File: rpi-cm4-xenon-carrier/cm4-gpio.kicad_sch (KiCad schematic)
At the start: 22 parts

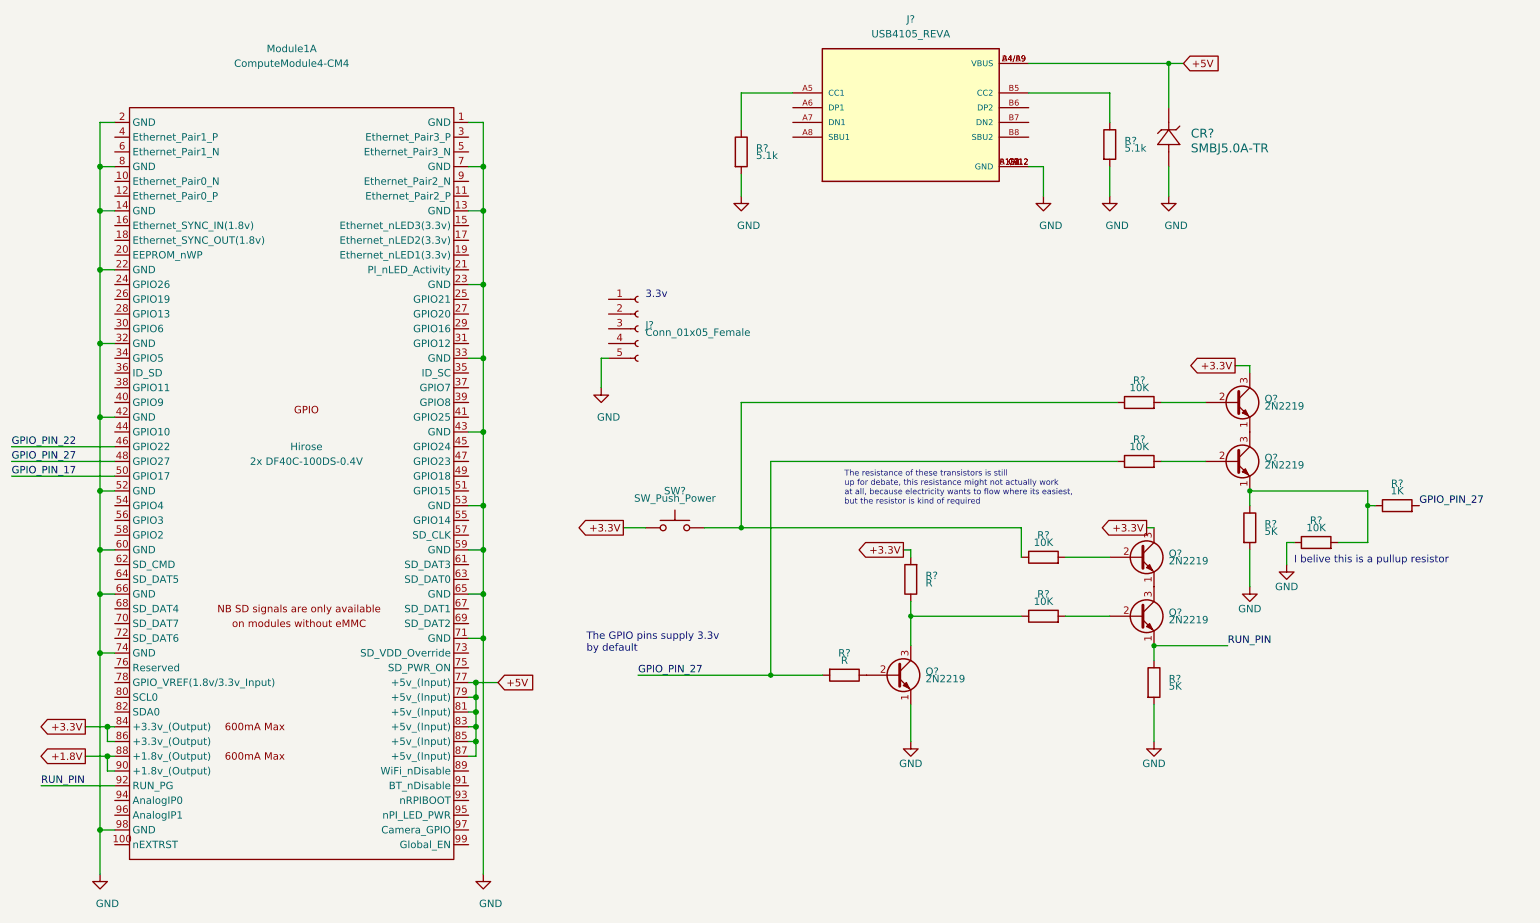
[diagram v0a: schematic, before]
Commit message: RP2040
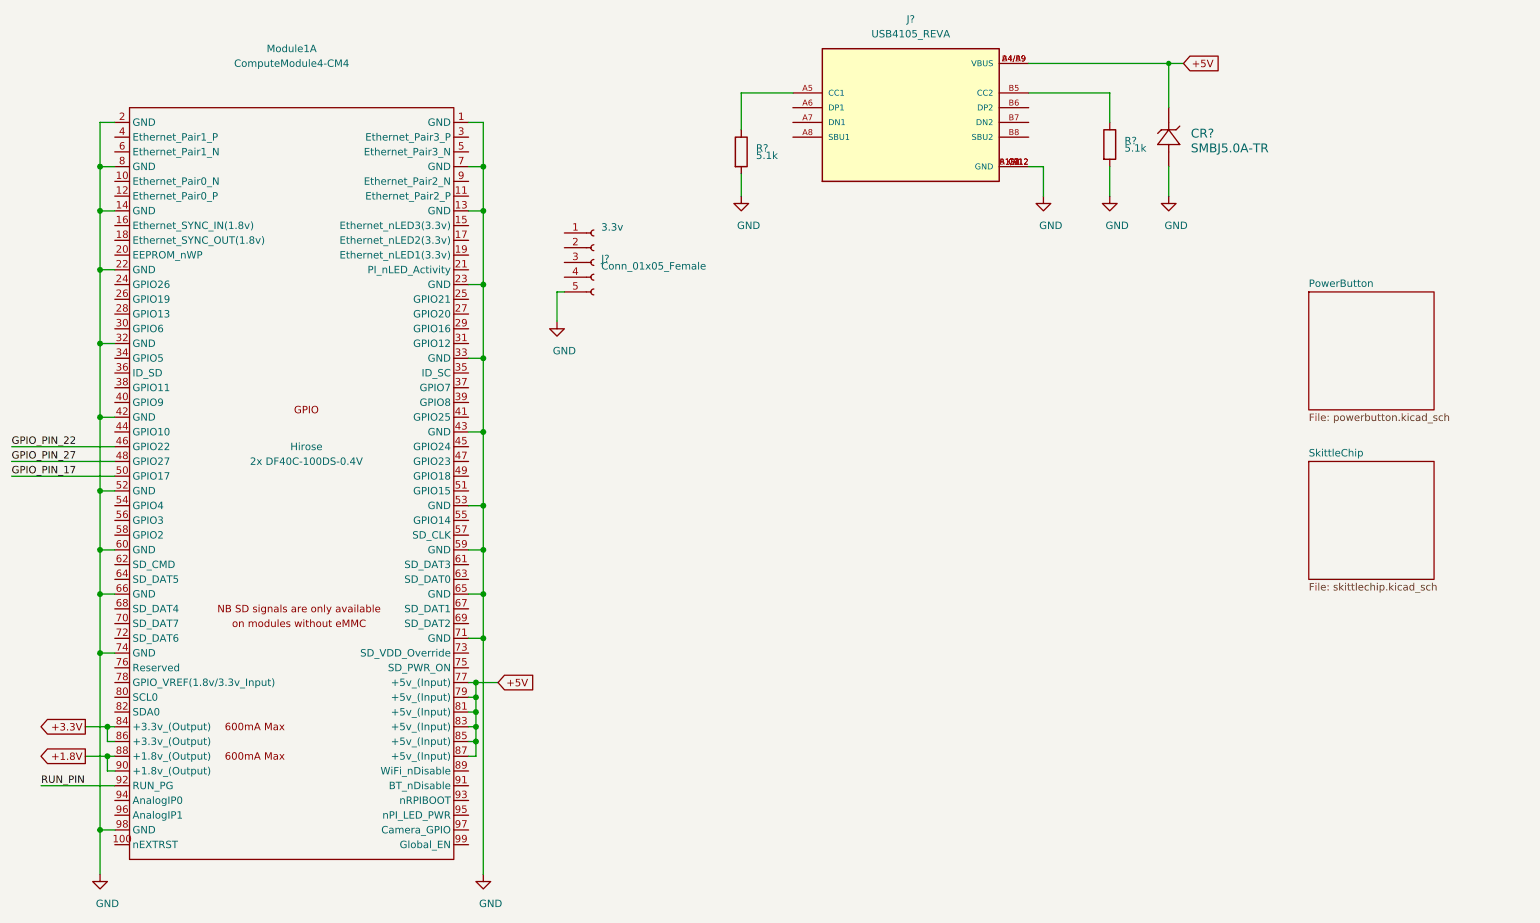
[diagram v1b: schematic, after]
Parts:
- removed Q? (x5): 2N2219, Package_TO_SOT_THT:TO-39-3, symbol Transistor_BJT:2N2219
- removed R? (x5): 10K, symbol Device:R
- removed R? (x2): 5K, symbol Device:R
- removed R? (x2): R, symbol Device:R
- removed R?: 1K, symbol Device:R
- removed SW?: SW_Push_Power, symbol Switch:SW_Push
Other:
- added sheet PowerButton (powerbutton.kicad_sch)
- added sheet SkittleChip (skittlechip.kicad_sch)
- note removed: "I belive this is a pullup resistor"
- note removed: "The GPIO pins supply 3.3v by default"
- note removed: "The resistance of these transistors is still up for debate, this resistance might not actually work at all, because electricity wants to flow where its easiest, but the resistor is kind of required"
- moved on the sheet: J?
